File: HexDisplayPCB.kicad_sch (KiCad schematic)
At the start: 79 parts, among them J1 Conn_01x20, J2 Conn_01x20, J3 Conn_01x16, J30 Barrel_Jack_Switch, J4 Conn_01x16, J5 Conn_01x16, J6 Conn_01x16, J7 Conn_01x16, J8 Conn_01x16, U1 SN74HCT245DWR

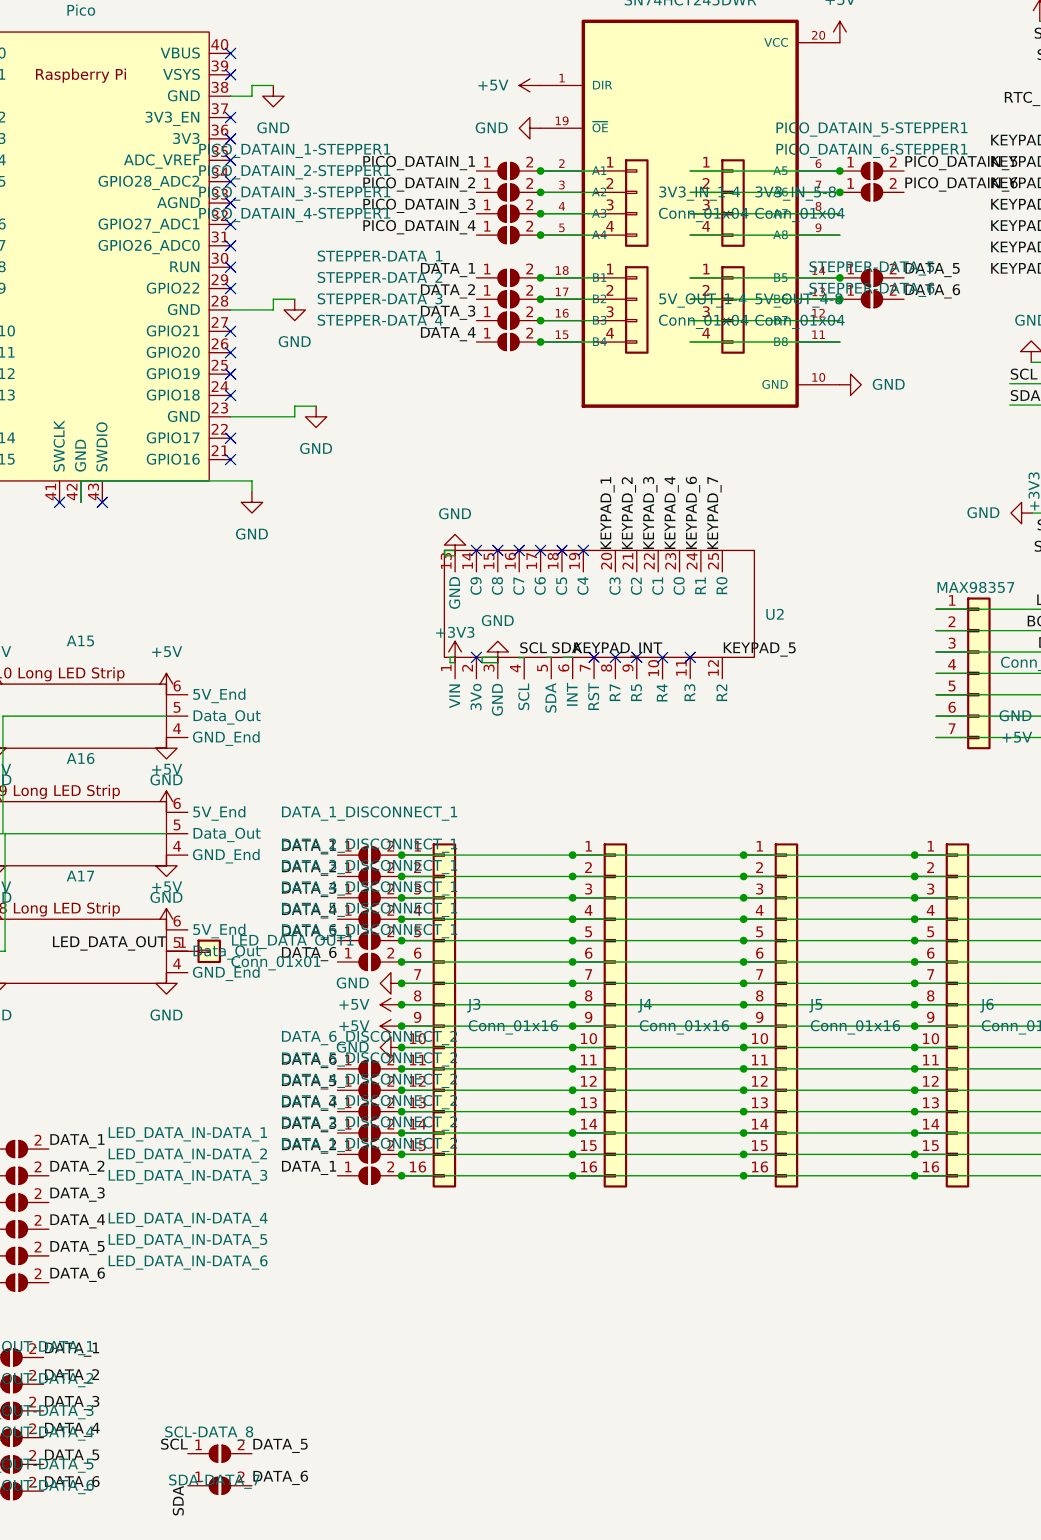
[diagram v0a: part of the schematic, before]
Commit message: Final first draft with gerber
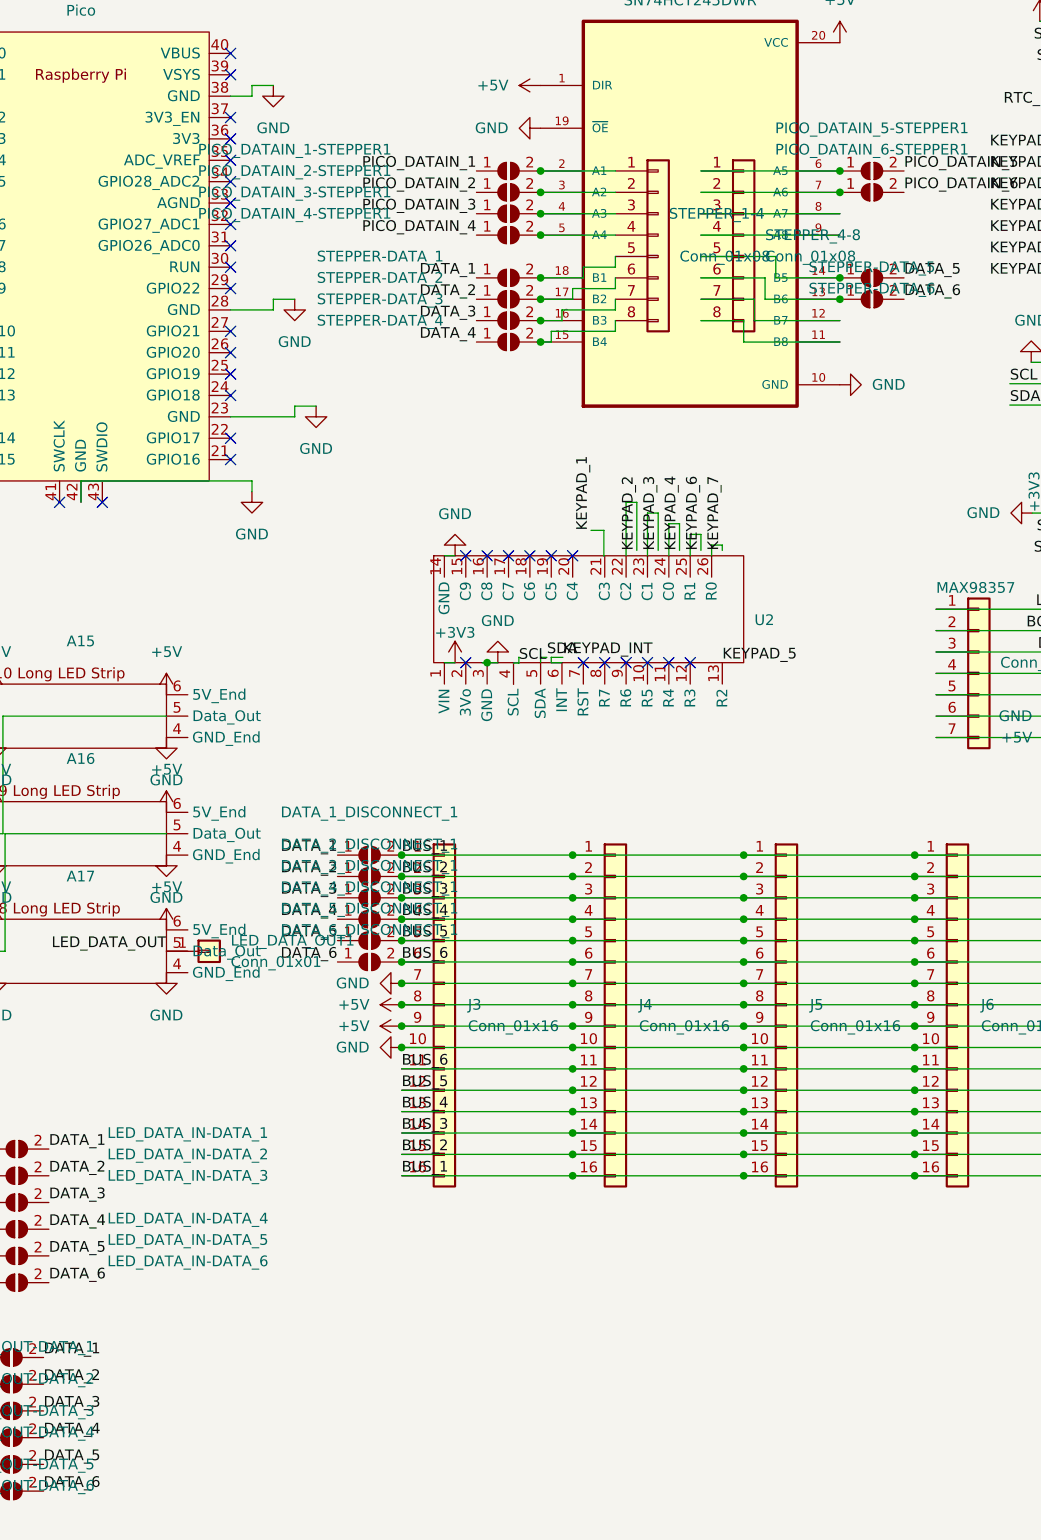
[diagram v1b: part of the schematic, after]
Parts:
- removed 3V3_IN_1-4, 3V3_IN_5-8, 5V_OUT_1-4, 5V_OUT_4-8: Conn_01x04, Connector_PinSocket_2.54mm:PinSocket_1x04_P2.54mm_Vertical, symbol Connector_Generic:Conn_01x04
- removed DATA_1_DISCONNECT_2, DATA_2_DISCONNECT_2, DATA_3_DISCONNECT_2, DATA_4_DISCONNECT_2, DATA_5_DISCONNECT_2, DATA_6_DISCONNECT_2, SCL-DATA_8, SDA-DATA_7: SolderJumper_2_Open, Jumper:SolderJumper-2_P1.3mm_Open_TrianglePad1.0x1.5mm, symbol Jumper:SolderJumper_2_Open
- added STEPPER_1-4, STEPPER_4-8: Conn_01x08, Connector_PinHeader_2.54mm:PinHeader_1x08_P2.54mm_Vertical, symbol Connector_Generic:Conn_01x08
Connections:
- net GND: now also U2.14 (GND); no longer U2.13 (GND)
- net KEYPAD_1: now also U2.21 (C3); no longer U2.20 (C3)
- net KEYPAD_2: now also U2.22 (C2); no longer U2.21 (C2)
- net KEYPAD_3: now also U2.23 (C1); no longer U2.22 (C1)
- net KEYPAD_4: now also U2.24 (C0); no longer U2.23 (C0)
- net KEYPAD_5: now also U2.13 (R2); no longer U2.12 (R2)
- net KEYPAD_6: now also U2.25 (R1); no longer U2.24 (R1)
- net KEYPAD_7: now also U2.26 (R0); no longer U2.25 (R0)
- net BUS_1: now reaches DATA_1_DISCONNECT_1.2 (B), J3.1 (Pin_1), J4.1 (Pin_1), J5.1 (Pin_1), J6.1 (Pin_1), J7.1 (Pin_1), J8.1 (Pin_1)
- net BUS_1: now also J3.16 (Pin_16), J4.16 (Pin_16), J5.16 (Pin_16), J6.16 (Pin_16), J7.16 (Pin_16), J8.16 (Pin_16)
- net BUS_6: now reaches J3.11 (Pin_11), J4.11 (Pin_11), J5.11 (Pin_11), J6.11 (Pin_11), J7.11 (Pin_11), J8.11 (Pin_11)
- net BUS_6: now also DATA_6_DISCONNECT_1.2 (B), J3.6 (Pin_6), J4.6 (Pin_6), J5.6 (Pin_6), J6.6 (Pin_6), J7.6 (Pin_6), J8.6 (Pin_6)
- net BUS_5: now reaches J3.12 (Pin_12), J4.12 (Pin_12), J5.12 (Pin_12), J6.12 (Pin_12), J7.12 (Pin_12), J8.12 (Pin_12)
- net BUS_5: now also DATA_5_DISCONNECT_1.2 (B), J3.5 (Pin_5), J4.5 (Pin_5), J5.5 (Pin_5), J6.5 (Pin_5), J7.5 (Pin_5), J8.5 (Pin_5)
- net BUS_4: now reaches J3.13 (Pin_13), J4.13 (Pin_13), J5.13 (Pin_13), J6.13 (Pin_13), J7.13 (Pin_13), J8.13 (Pin_13)
- net BUS_4: now also DATA_4_DISCONNECT_1.2 (B), J3.4 (Pin_4), J4.4 (Pin_4), J5.4 (Pin_4), J6.4 (Pin_4), J7.4 (Pin_4), J8.4 (Pin_4)
- net BUS_3: now reaches J3.14 (Pin_14), J4.14 (Pin_14), J5.14 (Pin_14), J6.14 (Pin_14), J7.14 (Pin_14), J8.14 (Pin_14)
- net BUS_3: now also DATA_3_DISCONNECT_1.2 (B), J3.3 (Pin_3), J4.3 (Pin_3), J5.3 (Pin_3), J6.3 (Pin_3), J7.3 (Pin_3), J8.3 (Pin_3)
- net BUS_2: now reaches J3.15 (Pin_15), J4.15 (Pin_15), J5.15 (Pin_15), J6.15 (Pin_15), J7.15 (Pin_15), J8.15 (Pin_15)
- net BUS_2: now also DATA_2_DISCONNECT_1.2 (B), J3.2 (Pin_2), J4.2 (Pin_2), J5.2 (Pin_2), J6.2 (Pin_2), J7.2 (Pin_2), J8.2 (Pin_2)
- net at PICO_DATAIN_1-STEPPER1.2 (B), U1.2 (A1): now also STEPPER_1-4.1 (Pin_1)
- net at PICO_DATAIN_2-STEPPER1.2 (B), U1.3 (A2): now also STEPPER_1-4.2 (Pin_2)
- net at PICO_DATAIN_3-STEPPER1.2 (B), U1.4 (A3): now also STEPPER_1-4.3 (Pin_3)
- net at PICO_DATAIN_4-STEPPER1.2 (B), U1.5 (A4): now also STEPPER_1-4.4 (Pin_4)
- net at STEPPER-DATA_5.1 (A), U1.14 (B5): now also STEPPER_4-8.5 (Pin_5)
- net at STEPPER-DATA_6.1 (A), U1.13 (B6): now also STEPPER_4-8.6 (Pin_6)
- net at U1.12 (B7): now also STEPPER_4-8.7 (Pin_7)
- net at U1.11 (B8): now also STEPPER_4-8.8 (Pin_8)
- net at PICO_DATAIN_5-STEPPER1.1 (A), U1.6 (A5): now also STEPPER_4-8.1 (Pin_1)
- net at PICO_DATAIN_6-STEPPER1.1 (A), U1.7 (A6): now also STEPPER_4-8.2 (Pin_2)
- net at U1.8 (A7): now also STEPPER_4-8.3 (Pin_3)
- net at U1.9 (A8): now also STEPPER_4-8.4 (Pin_4)
- net at STEPPER-DATA_4.2 (B), U1.15 (B4): now also STEPPER_1-4.8 (Pin_8)
- net at STEPPER-DATA_3.2 (B), U1.16 (B3): now also STEPPER_1-4.7 (Pin_7)
- net at STEPPER-DATA_2.2 (B), U1.17 (B2): now also STEPPER_1-4.6 (Pin_6)
- net at STEPPER-DATA_1.2 (B), U1.18 (B1): now also STEPPER_1-4.5 (Pin_5)
- no-connect marks 46 -> 47

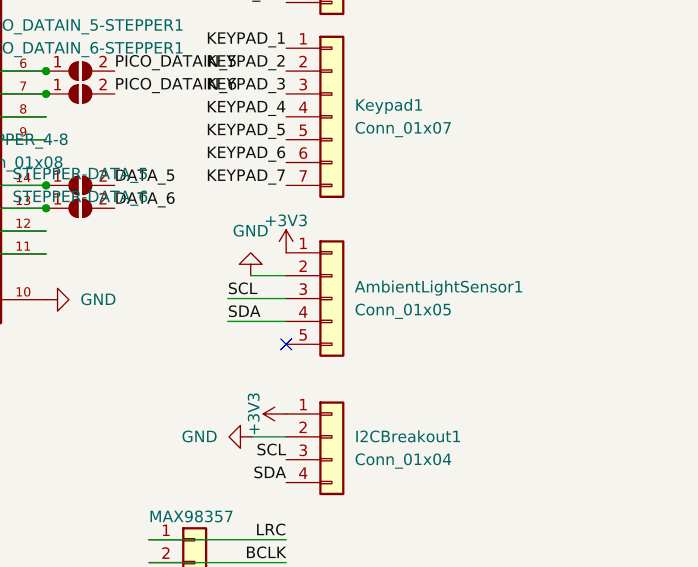
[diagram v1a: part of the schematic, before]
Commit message: Final image adjustments
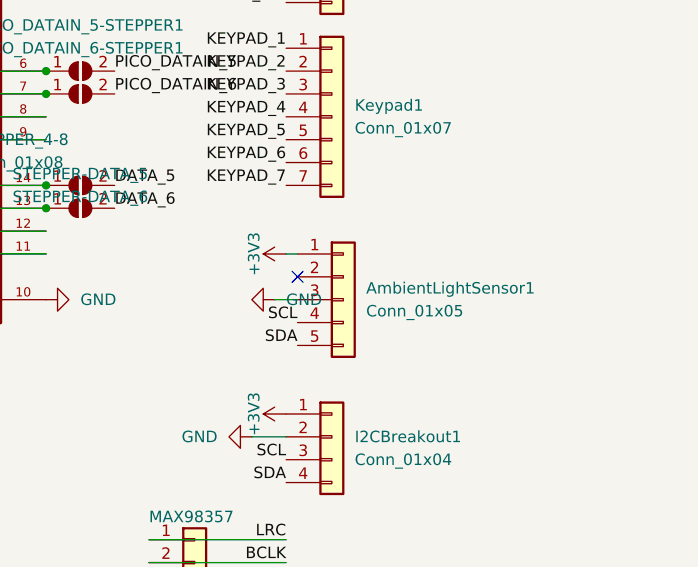
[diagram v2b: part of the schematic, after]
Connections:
- net GND: now also AmbientLightSensor1.3 (Pin_3); no longer AmbientLightSensor1.2 (Pin_2)
- net SCL: now also AmbientLightSensor1.4 (Pin_4); no longer AmbientLightSensor1.3 (Pin_3)
- net SDA: now also AmbientLightSensor1.5 (Pin_5); no longer AmbientLightSensor1.4 (Pin_4)
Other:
- moved on the sheet: AmbientLightSensor1
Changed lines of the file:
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@@
   (no_connect (at 165.1 31.75))
   (no_connect (at 165.1 24.13))
-  (no_connect (at 264.16 68.453))
+  (no_connect (at 265.43 60.96))
   (no_connect (at 212.09 96.52))
   (no_connect (at 165.1 44.45))
@@
     (stroke (width 0) (type default))
   )
-  (wire (pts (xy 257.683 63.373) (xy 264.16 63.373))
-    (stroke (width 0) (type default))
-  )
   (wire (pts (xy 205.74 157.48) (xy 226.06 157.48))
     (stroke (width 0) (type default))
@@
     (stroke (width 0) (type default))
   )
-  (wire (pts (xy 260.223 60.833) (xy 264.16 60.833))
-    (stroke (width 0) (type default))
-  )
   (wire (pts (xy 91.44 40.64) (xy 93.98 40.64))
     (stroke (width 0) (type default))
   )
-  (wire (pts (xy 257.683 65.913) (xy 264.16 65.913))
-    (stroke (width 0) (type default))
-  )
   (wire (pts (xy 226.06 157.48) (xy 246.38 157.48))
     (stroke (width 0) (type default))
@@
     (stroke (width 0) (type default))
   )
+  (wire (pts (xy 262.89 63.5) (xy 265.43 63.5))
+    (stroke (width 0) (type default))
+  )
   (wire (pts (xy 46.99 48.26) (xy 55.88 48.26))
     (stroke (width 0) (type default))
@@
     (stroke (width 0) (type default))
   )
+  (wire (pts (xy 264.16 58.42) (xy 265.43 58.42))
+    (stroke (width 0) (type default))
+  )
   (wire (pts (xy 226.06 144.78) (xy 246.38 144.78))
     (stroke (width 0) (type default))
@@
     (effects (font (size 1.27 1.27)) (justify left bottom))
   )
-  (label "SCL" (at 257.683 63.373 0) (fields_autoplaced)
-    (effects (font (size 1.27 1.27)) (justify left bottom))
-  )
   (label "DATA_5" (at 245.11 50.8 0) (fields_autoplaced)
     (effects (font (size 1.27 1.27)) (justify left bottom))
@@
     (effects (font (size 1.27 1.27)) (justify left bottom))
   )
+  (label "SDA" (at 265.43 68.58 180) (fields_autoplaced)
+    (effects (font (size 1.27 1.27)) (justify right bottom))
+  )
   (label "LRC" (at 46.99 30.48 0) (fields_autoplaced)
     (effects (font (size 1.27 1.27)) (justify left bottom))
@@
     (effects (font (size 1.27 1.27)) (justify right bottom))
   )
-  (label "SDA" (at 257.683 65.913 0) (fields_autoplaced)
-    (effects (font (size 1.27 1.27)) (justify left bottom))
-  )
   (label "KEYPAD_5" (at 223.52 96.52 0) (fields_autoplaced)
     (effects (font (size 1.27 1.27)) (justify left bottom))
@@
     (effects (font (size 1.27 1.27)) (justify left bottom))
   )
+  (label "SCL" (at 265.43 66.04 180) (fields_autoplaced)
+    (effects (font (size 1.27 1.27)) (justify right bottom))
+  )
   (label "PICO_DATAIN_2" (at 46.99 58.42 0) (fields_autoplaced)
     (effects (font (size 1.27 1.27)) (justify left bottom))
@@
     )
   )
-  (symbol (lib_id "power:+3V3") (at 264.16 58.293 0) (unit 1)
+  (symbol (lib_id "power:+3V3") (at 264.16 58.42 90) (unit 1)
     (in_bom yes) (on_board yes) (dnp no)
-    (property "Reference" "#PWR087" (at 264.16 62.103 0)
+    (property "Reference" "#PWR087" (at 267.97 58.42 0)
       (effects (font (size 1.27 1.27)) hide)
     )
-    (property "Value" "+3V3" (at 264.16 54.737 0)
+    (property "Value" "+3V3" (at 260.604 58.42 0)
       (effects (font (size 1.27 1.27)))
     )
-    (property "Footprint" "" (at 264.16 58.293 0)
+    (property "Footprint" "" (at 264.16 58.42 0)
       (effects (font (size 1.27 1.27)) hide)
     )
-    (property "Datasheet" "" (at 264.16 58.293 0)
+    (property "Datasheet" "" (at 264.16 58.42 0)
       (effects (font (size 1.27 1.27)) hide)
     )
@@
     )
   )
-  (symbol (lib_id "Connector_Generic:Conn_01x05") (at 269.24 63.373 0) (unit 1)
+  (symbol (lib_id "Connector_Generic:Conn_01x05") (at 270.51 63.5 0) (unit 1)
     (in_bom yes) (on_board yes) (dnp no) (fields_autoplaced)
-    (property "Reference" "AmbientLightSensor1" (at 271.78 62.103 0)
+    (property "Reference" "AmbientLightSensor1" (at 273.05 62.23 0)
       (effects (font (size 1.27 1.27)) (justify left))
     )
-    (property "Value" "Conn_01x05" (at 271.78 64.643 0)
+    (property "Value" "Conn_01x05" (at 273.05 64.77 0)
       (effects (font (size 1.27 1.27)) (justify left))
     )
-    (property "Footprint" "Connector_PinHeader_2.54mm:PinHeader_1x05_P2.54mm_Vertical" (at 269.24 63.373 0)
+    (property "Footprint" "Connector_PinHeader_2.54mm:PinHeader_1x05_P2.54mm_Vertical" (at 270.51 63.5 0)
       (effects (font (size 1.27 1.27)) hide)
     )
-    (property "Datasheet" "~" (at 269.24 63.373 0)
+    (property "Datasheet" "~" (at 270.51 63.5 0)
       (effects (font (size 1.27 1.27)) hide)
     )
@@
     )
   )
-  (symbol (lib_id "power:GND") (at 260.223 60.833 180) (unit 1)
+  (symbol (lib_id "power:GND") (at 262.89 63.5 270) (unit 1)
     (in_bom yes) (on_board yes) (dnp no) (fields_autoplaced)
-    (property "Reference" "#PWR086" (at 260.223 54.483 0)
+    (property "Reference" "#PWR086" (at 256.54 63.5 0)
       (effects (font (size 1.27 1.27)) hide)
     )
-    (property "Value" "GND" (at 260.223 55.88 0)
-      (effects (font (size 1.27 1.27)))
+    (property "Value" "GND" (at 264.16 63.5 90)
+      (effects (font (size 1.27 1.27)) (justify left))
     )
-    (property "Footprint" "" (at 260.223 60.833 0)
+    (property "Footprint" "" (at 262.89 63.5 0)
       (effects (font (size 1.27 1.27)) hide)
     )
-    (property "Datasheet" "" (at 260.223 60.833 0)
+    (property "Datasheet" "" (at 262.89 63.5 0)
       (effects (font (size 1.27 1.27)) hide)
     )
